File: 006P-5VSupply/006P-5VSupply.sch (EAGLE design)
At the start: 14 parts, among them IC1 7805T

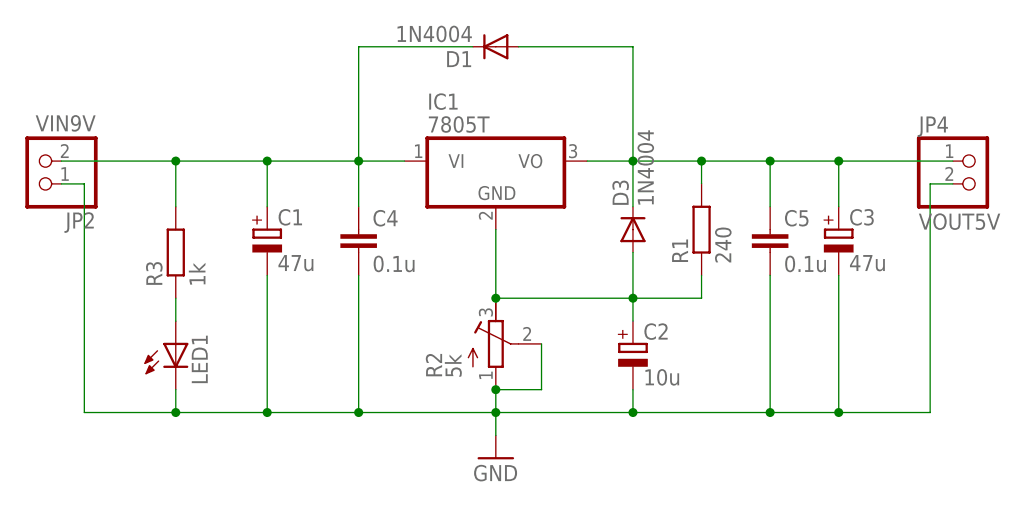
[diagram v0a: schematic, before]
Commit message: Update 006P-5VSupply Project
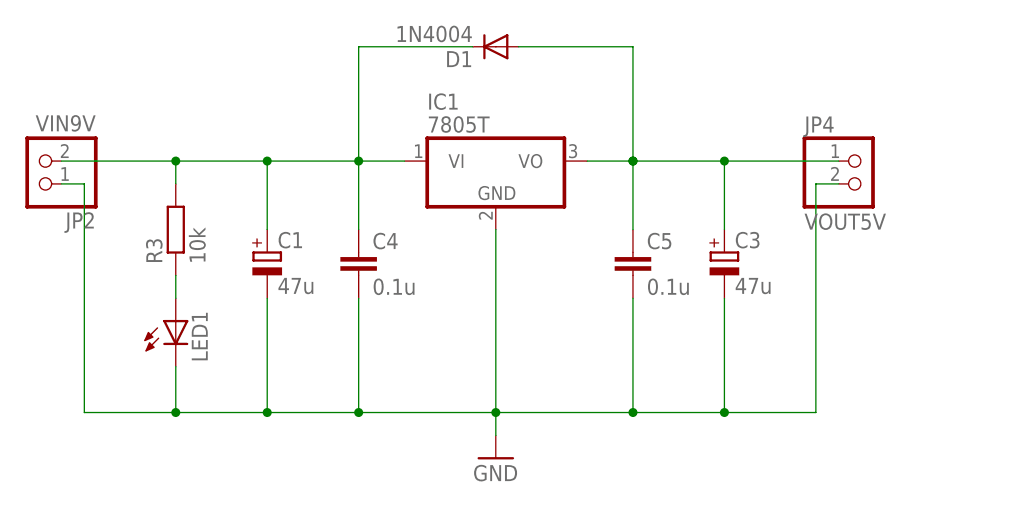
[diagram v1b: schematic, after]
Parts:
- removed C2: 10u, rcl:CPOL-EUE2-4
- removed D3: 1N4004, diode:1N4004
- removed R1: 240, rcl:R-EU_0207/7
- removed R2: 5k, rcl:R-TRIMM3339P
- R3: value 1k -> 10k
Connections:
- removed net N$3: C2.+, D3.A, IC1.GND, R1.1, R2.E
- net GND: now also IC1.GND; no longer C2.-, R2.A, R2.S
- net N$1: no longer D3.C, R1.2
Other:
- moved on the sheet: C1, C3, C4, C5, JP4, LED1, R3
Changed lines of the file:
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@@
 <setting verticaltext="up"/>
 </settings>
-<grid distance="0.1" unitdist="inch" unit="inch" style="dots" multiple="1" display="yes" altdistance="0.01" altunitdist="inch" altunit="inch"/>
+<grid distance="0.1" unitdist="inch" unit="inch" style="lines" multiple="1" display="no" altdistance="0.01" altunitdist="inch" altunit="inch"/>
 <layers>
 <layer number="1" name="Top" color="4" fill="1" visible="no" active="no"/>
@@
 <parts>
 <part name="IC1" library="linear" deviceset="78*" device="T" technology="05"/>
-<part name="R1" library="rcl" deviceset="R-EU_" device="0207/7" value="240"/>
 <part name="D1" library="diode" deviceset="1N4004" device=""/>
-<part name="D3" library="diode" deviceset="1N4004" device=""/>
 <part name="C1" library="rcl" deviceset="CPOL-EU" device="E2-4" value="47u"/>
-<part name="C2" library="rcl" deviceset="CPOL-EU" device="E2-4" value="10u"/>
 <part name="C3" library="rcl" deviceset="CPOL-EU" device="E2-4" value="47u"/>
 <part name="C4" library="rcl" deviceset="C-EU" device="025-024X044" value="0.1u"/>
@@
 <part name="JP4" library="pinhead" deviceset="PINHD-1X2" device="" value="VOUT5V"/>
 <part name="LED1" library="led" deviceset="LED" device="3MM"/>
-<part name="R2" library="rcl" deviceset="R-TRIMM" device="3339P" value="5k"/>
-<part name="R3" library="rcl" deviceset="R-EU_" device="0207/7" value="1k"/>
+<part name="R3" library="rcl" deviceset="R-EU_" device="0207/7" value="10k"/>
 </parts>
 <sheets>
@@
 <instances>
 <instance part="IC1" gate="A1" x="58.42" y="73.66"/>
-<instance part="R1" gate="G$1" x="81.28" y="66.04" rot="R90"/>
 <instance part="D1" gate="1" x="58.42" y="86.36" rot="R180"/>
-<instance part="D3" gate="1" x="73.66" y="66.04" rot="R90"/>
-<instance part="C1" gate="G$1" x="33.02" y="66.04"/>
-<instance part="C2" gate="G$1" x="73.66" y="53.34"/>
-<instance part="C3" gate="G$1" x="96.52" y="66.04"/>
-<instance part="C4" gate="G$1" x="43.18" y="66.04"/>
-<instance part="C5" gate="G$1" x="88.9" y="66.04"/>
+<instance part="C1" gate="G$1" x="33.02" y="63.5"/>
+<instance part="C3" gate="G$1" x="83.82" y="63.5"/>
+<instance part="C4" gate="G$1" x="43.18" y="63.5"/>
+<instance part="C5" gate="G$1" x="73.66" y="63.5"/>
 <instance part="GND1" gate="1" x="58.42" y="40.64"/>
 <instance part="JP2" gate="G$1" x="7.62" y="73.66" rot="R180"/>
-<instance part="JP4" gate="G$1" x="111.76" y="71.12"/>
-<instance part="LED1" gate="G$1" x="22.86" y="53.34"/>
-<instance part="R2" gate="G$1" x="58.42" y="53.34"/>
-<instance part="R3" gate="G$1" x="22.86" y="63.5" rot="R90"/>
+<instance part="JP4" gate="G$1" x="99.06" y="71.12"/>
+<instance part="LED1" gate="G$1" x="22.86" y="55.88"/>
+<instance part="R3" gate="G$1" x="22.86" y="66.04" rot="R90"/>
 </instances>
 <busses>
@@
 <pinref part="IC1" gate="A1" pin="VO"/>
 <wire x1="68.58" y1="73.66" x2="73.66" y2="73.66" width="0.1524" layer="91"/>
-<pinref part="D3" gate="1" pin="C"/>
-<wire x1="73.66" y1="73.66" x2="73.66" y2="68.58" width="0.1524" layer="91"/>
-<pinref part="R1" gate="G$1" pin="2"/>
-<wire x1="81.28" y1="71.12" x2="81.28" y2="73.66" width="0.1524" layer="91"/>
-<wire x1="81.28" y1="73.66" x2="73.66" y2="73.66" width="0.1524" layer="91"/>
 <junction x="73.66" y="73.66"/>
 <pinref part="C5" gate="G$1" pin="1"/>
-<wire x1="88.9" y1="68.58" x2="88.9" y2="73.66" width="0.1524" layer="91"/>
-<wire x1="88.9" y1="73.66" x2="81.28" y2="73.66" width="0.1524" layer="91"/>
-<junction x="81.28" y="73.66"/>
+<wire x1="73.66" y1="66.04" x2="73.66" y2="73.66" width="0.1524" layer="91"/>
 <pinref part="C3" gate="G$1" pin="+"/>
-<wire x1="88.9" y1="73.66" x2="96.52" y2="73.66" width="0.1524" layer="91"/>
-<wire x1="96.52" y1="73.66" x2="96.52" y2="68.58" width="0.1524" layer="91"/>
-<junction x="88.9" y="73.66"/>
+<wire x1="73.66" y1="73.66" x2="83.82" y2="73.66" width="0.1524" layer="91"/>
+<wire x1="83.82" y1="73.66" x2="83.82" y2="66.04" width="0.1524" layer="91"/>
+<junction x="73.66" y="73.66"/>
 <pinref part="D1" gate="1" pin="A"/>
 <wire x1="60.96" y1="86.36" x2="73.66" y2="86.36" width="0.1524" layer="91"/>
 <wire x1="73.66" y1="86.36" x2="73.66" y2="73.66" width="0.1524" layer="91"/>
 <pinref part="JP4" gate="G$1" pin="1"/>
-<wire x1="96.52" y1="73.66" x2="109.22" y2="73.66" width="0.1524" layer="91"/>
-<junction x="96.52" y="73.66"/>
-</segment>
-</net>
-<net name="N$3" class="0">
-<segment>
-<pinref part="IC1" gate="A1" pin="GND"/>
-<wire x1="58.42" y1="66.04" x2="58.42" y2="58.42" width="0.1524" layer="91"/>
-<wire x1="58.42" y1="58.42" x2="73.66" y2="58.42" width="0.1524" layer="91"/>
-<pinref part="R1" gate="G$1" pin="1"/>
-<wire x1="73.66" y1="58.42" x2="81.28" y2="58.42" width="0.1524" layer="91"/>
-<wire x1="81.28" y1="58.42" x2="81.28" y2="60.96" width="0.1524" layer="91"/>
-<pinref part="D3" gate="1" pin="A"/>
-<wire x1="73.66" y1="63.5" x2="73.66" y2="58.42" width="0.1524" layer="91"/>
-<junction x="73.66" y="58.42"/>
-<pinref part="C2" gate="G$1" pin="+"/>
-<wire x1="73.66" y1="58.42" x2="73.66" y2="55.88" width="0.1524" layer="91"/>
-<pinref part="R2" gate="G$1" pin="E"/>
-<junction x="58.42" y="58.42"/>
+<wire x1="83.82" y1="73.66" x2="96.52" y2="73.66" width="0.1524" layer="91"/>
+<junction x="83.82" y="73.66"/>
 </segment>
 </net>
@@
 <segment>
 <pinref part="C1" gate="G$1" pin="+"/>
-<wire x1="33.02" y1="68.58" x2="33.02" y2="73.66" width="0.1524" layer="91"/>
+<wire x1="33.02" y1="66.04" x2="33.02" y2="73.66" width="0.1524" layer="91"/>
 <pinref part="IC1" gate="A1" pin="VI"/>
 <wire x1="33.02" y1="73.66" x2="43.18" y2="73.66" width="0.1524" layer="91"/>
 <wire x1="43.18" y1="73.66" x2="48.26" y2="73.66" width="0.1524" layer="91"/>
 <pinref part="C4" gate="G$1" pin="1"/>
-<wire x1="43.18" y1="68.58" x2="43.18" y2="73.66" width="0.1524" layer="91"/>
+<wire x1="43.18" y1="66.04" x2="43.18" y2="73.66" width="0.1524" layer="91"/>
 <junction x="43.18" y="73.66"/>
 <wire x1="43.18" y1="73.66" x2="43.18" y2="86.36" width="0.1524" layer="91"/>
@@
 <pinref part="R3" gate="G$1" pin="2"/>
 <wire x1="22.86" y1="73.66" x2="33.02" y2="73.66" width="0.1524" layer="91"/>
-<wire x1="22.86" y1="68.58" x2="22.86" y2="73.66" width="0.1524" layer="91"/>
+<wire x1="22.86" y1="71.12" x2="22.86" y2="73.66" width="0.1524" layer="91"/>
 <junction x="22.86" y="73.66"/>
 </segment>
@@
 <pinref part="C1" gate="G$1" pin="-"/>
 <wire x1="58.42" y1="45.72" x2="58.42" y2="43.18" width="0.1524" layer="91"/>
-<wire x1="33.02" y1="60.96" x2="33.02" y2="45.72" width="0.1524" layer="91"/>
+<wire x1="33.02" y1="58.42" x2="33.02" y2="45.72" width="0.1524" layer="91"/>
 <wire x1="33.02" y1="45.72" x2="43.18" y2="45.72" width="0.1524" layer="91"/>
 <junction x="58.42" y="45.72"/>
 <wire x1="43.18" y1="45.72" x2="58.42" y2="45.72" width="0.1524" layer="91"/>
 <pinref part="C4" gate="G$1" pin="2"/>
-<wire x1="43.18" y1="60.96" x2="43.18" y2="45.72" width="0.1524" layer="91"/>
+<wire x1="43.18" y1="58.42" x2="43.18" y2="45.72" width="0.1524" layer="91"/>
 <junction x="43.18" y="45.72"/>
+<pinref part="C3" gate="G$1" pin="-"/>
 <wire x1="58.42" y1="45.72" x2="73.66" y2="45.72" width="0.1524" layer="91"/>
-<pinref part="C2" gate="G$1" pin="-"/>
-<wire x1="73.66" y1="45.72" x2="73.66" y2="48.26" width="0.1524" layer="91"/>
-<pinref part="C3" gate="G$1" pin="-"/>
-<wire x1="73.66" y1="45.72" x2="88.9" y2="45.72" width="0.1524" layer="91"/>
-<wire x1="88.9" y1="45.72" x2="96.52" y2="45.72" width="0.1524" layer="91"/>
-<wire x1="96.52" y1="45.72" x2="96.52" y2="60.96" width="0.1524" layer="91"/>
+<wire x1="73.66" y1="45.72" x2="83.82" y2="45.72" width="0.1524" layer="91"/>
+<wire x1="83.82" y1="45.72" x2="83.82" y2="58.42" width="0.1524" layer="91"/>
+<pinref part="C5" gate="G$1" pin="2"/>
+<wire x1="73.66" y1="58.42" x2="73.66" y2="45.72" width="0.1524" layer="91"/>
 <junction x="73.66" y="45.72"/>
-<pinref part="C5" gate="G$1" pin="2"/>
-<wire x1="88.9" y1="60.96" x2="88.9" y2="45.72" width="0.1524" layer="91"/>
-<junction x="88.9" y="45.72"/>
 <pinref part="JP2" gate="G$1" pin="1"/>
 <wire x1="10.16" y1="71.12" x2="12.7" y2="71.12" width="0.1524" layer="91"/>
@@
 <pinref part="JP4" gate="G$1" pin="2"/>
 <wire x1="22.86" y1="45.72" x2="33.02" y2="45.72" width="0.1524" layer="91"/>
-<wire x1="109.22" y1="71.12" x2="106.68" y2="71.12" width="0.1524" layer="91"/>
-<wire x1="106.68" y1="71.12" x2="106.68" y2="45.72" width="0.1524" layer="91"/>
-<wire x1="106.68" y1="45.72" x2="96.52" y2="45.72" width="0.1524" layer="91"/>
-<junction x="96.52" y="45.72"/>
+<wire x1="96.52" y1="71.12" x2="93.98" y2="71.12" width="0.1524" layer="91"/>
+<wire x1="93.98" y1="71.12" x2="93.98" y2="45.72" width="0.1524" layer="91"/>
+<wire x1="93.98" y1="45.72" x2="83.82" y2="45.72" width="0.1524" layer="91"/>
+<junction x="83.82" y="45.72"/>
 <pinref part="LED1" gate="G$1" pin="C"/>
-<wire x1="22.86" y1="48.26" x2="22.86" y2="45.72" width="0.1524" layer="91"/>
+<wire x1="22.86" y1="50.8" x2="22.86" y2="45.72" width="0.1524" layer="91"/>
 <junction x="22.86" y="45.72"/>
-<pinref part="R2" gate="G$1" pin="A"/>
-<wire x1="58.42" y1="45.72" x2="58.42" y2="48.26" width="0.1524" layer="91"/>
-<pinref part="R2" gate="G$1" pin="S"/>
-<wire x1="63.5" y1="53.34" x2="63.5" y2="48.26" width="0.1524" layer="91"/>
-<wire x1="63.5" y1="48.26" x2="58.42" y2="48.26" width="0.1524" layer="91"/>
-<junction x="58.42" y="48.26"/>
+<pinref part="IC1" gate="A1" pin="GND"/>
+<wire x1="58.42" y1="66.04" x2="58.42" y2="45.72" width="0.1524" layer="91"/>
 </segment>
 </net>
@@
 <pinref part="R3" gate="G$1" pin="1"/>
 <pinref part="LED1" gate="G$1" pin="A"/>
-<wire x1="22.86" y1="58.42" x2="22.86" y2="55.88" width="0.1524" layer="91"/>
+<wire x1="22.86" y1="60.96" x2="22.86" y2="58.42" width="0.1524" layer="91"/>
 </segment>
 </net>
